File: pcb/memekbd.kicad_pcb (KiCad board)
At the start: 2 copper layers, 341 x 293.4 mm, 235 parts, among them J1 AudioJack4, J2 AudioJack4, SW1 SW_Push, SW10 SW_Push, SW11 SW_Push, SW12 SW_Push, SW13 SW_Push, SW14 SW_Push, SW15 SW_Push, SW16 SW_Push, SW17 SW_Push, SW18 SW_Push, SW19 SW_Push, SW2 SW_Push, SW20 SW_Push, SW21 SW_Push, SW22 SW_Push, SW23 SW_Push, SW24 SW_Push, SW25 SW_Push, SW26 SW_Push, SW27 SW_Push, SW28 SW_Push, SW29 SW_Push, SW3 SW_Push, SW30 SW_Push, SW31 SW_Push, SW32 SW_Push, SW33 SW_Push, SW34 SW_Push, SW35 SW_Push, SW36 SW_Push, SW37 SW_Push, SW38 SW_Push, SW39 SW_Push, SW4 SW_Push, SW40 SW_Push, SW41 SW_Push, SW42 SW_Push, SW43 SW_Push, SW44 SW_Push, SW45 SW_Push, SW46 SW_Push, SW47 SW_Push, SW48 SW_Push, SW5 SW_Push, SW6 SW_Push, SW7 SW_Push, SW8 SW_Push, SW9 SW_Push, U1 ProMicro, U2 ProMicro

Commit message: Pcb progress
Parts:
- moved C19 3.95 mm to (126.5, 114.3)
- moved C1 3.95 mm to (27.0, 52.2)
- moved C10 3.95 mm to (64.5, 19.2)
- moved C11 3.95 mm to (64.5, 38.8)
- moved C12 3.95 mm to (64.5, 57.2)
- moved C13 3.95 mm to (64.5, 76.8)
- moved C14 3.95 mm to (102.5, 102.3)
- moved C15 3.95 mm to (83.0, 26.2)
- moved C16 3.95 mm to (83.0, 45.8)
- moved C17 3.95 mm to (83.0, 64.2)
- moved C18 3.95 mm to (83.5, 83.2)
- moved C2 3.95 mm to (27.0, 71.2)
- moved C20 3.95 mm to (103.0, 45.2)
- moved C21 3.95 mm to (102.5, 64.8)
- moved C22 3.95 mm to (102.0, 83.2)
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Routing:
- net +5V: track 1560.0 -> 1413.5 mm
- net /rcol3: track 0.00 -> 113.6 mm
- net /rcol1: track 0.00 -> 111.0 mm
- net /rcol2: track 0.00 -> 108.8 mm
- net /rcol0: track 0.00 -> 94.2 mm
- net /rrow1: track 0.00 -> 92.9 mm, vias 0 -> 8
- net /rrow2: track 0.00 -> 91.2 mm, vias 0 -> 7
- net /rrow3: track 0.00 -> 88.8 mm, vias 0 -> 3
- net /rcol4: track 0.00 -> 84.2 mm
- net /rrow4: track 0.00 -> 78.4 mm
- net /rrow0: track 0.00 -> 71.0 mm
- net GND: track 1293.3 -> 1223.3 mm
- net Net-(LED24-Pad4): track 0.00 -> 22.0 mm
- net Net-(LED28-Pad4): track 0.00 -> 9.37 mm
- net Net-(D42-Pad2): track 0.00 -> 4.40 mm
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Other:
- board size 341 x 293.4 mm -> 344.8 x 294.6 mm

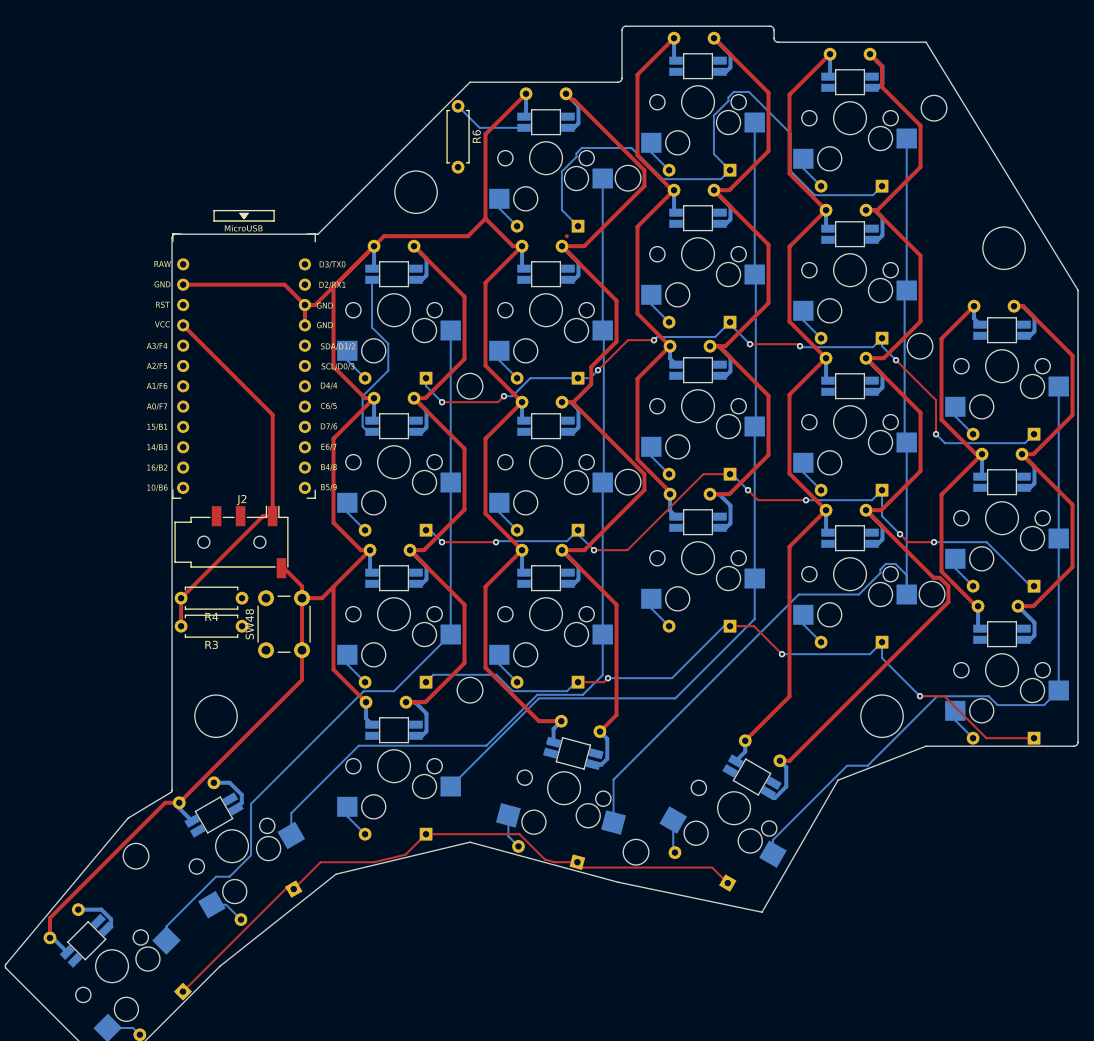
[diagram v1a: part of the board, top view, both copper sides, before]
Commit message: Pcb progress
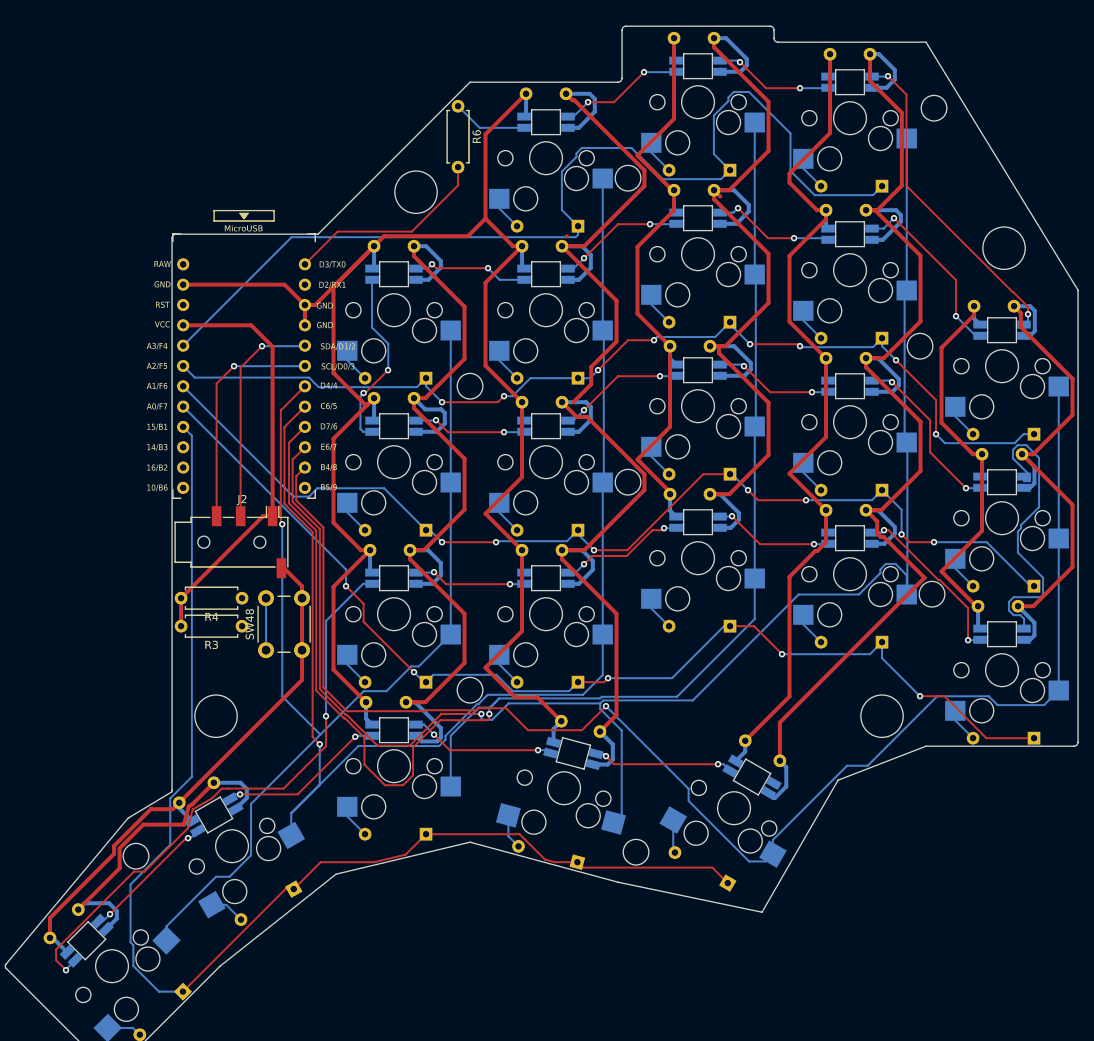
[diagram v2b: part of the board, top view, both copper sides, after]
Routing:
- net /rcol4: track 84.2 -> 182.8 mm, vias 0 -> 1
- net +5V: track 1413.5 -> 1496.7 mm
- net /rcol3: track 113.6 -> 195.9 mm, vias 0 -> 1
- net /rrow4: track 78.4 -> 157.1 mm
- net /rcol2: track 108.8 -> 184.8 mm, vias 0 -> 1
- net Net-(LED26-Pad4): track 0.00 -> 73.1 mm, vias 0 -> 2
- net /rrow0: track 71.0 -> 127.1 mm
- net /rcol1: track 111.0 -> 166.5 mm, vias 0 -> 1
- net /rrow3: track 88.8 -> 136.0 mm, vias 3 -> 5
- net /rcol0: track 94.2 -> 141.0 mm, vias 0 -> 1
- net Net-(LED38-Pad2): track 0.00 -> 40.6 mm, vias 0 -> 2
- net Net-(LED44-Pad2): track 0.00 -> 39.0 mm
- net /rrow2: track 91.2 -> 129.8 mm
- net /rrow1: track 92.9 -> 124.8 mm
- net /rSCL: track 0.00 -> 28.5 mm, vias 0 -> 1
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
